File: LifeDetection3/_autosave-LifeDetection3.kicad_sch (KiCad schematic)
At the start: 21 parts, among them J1 Power, J12 XT60PW-M, J2 PWM, J3 Analog, J4 PWM, J5 Analog, J6 Communication, J7 Digital, U1 TLP3545

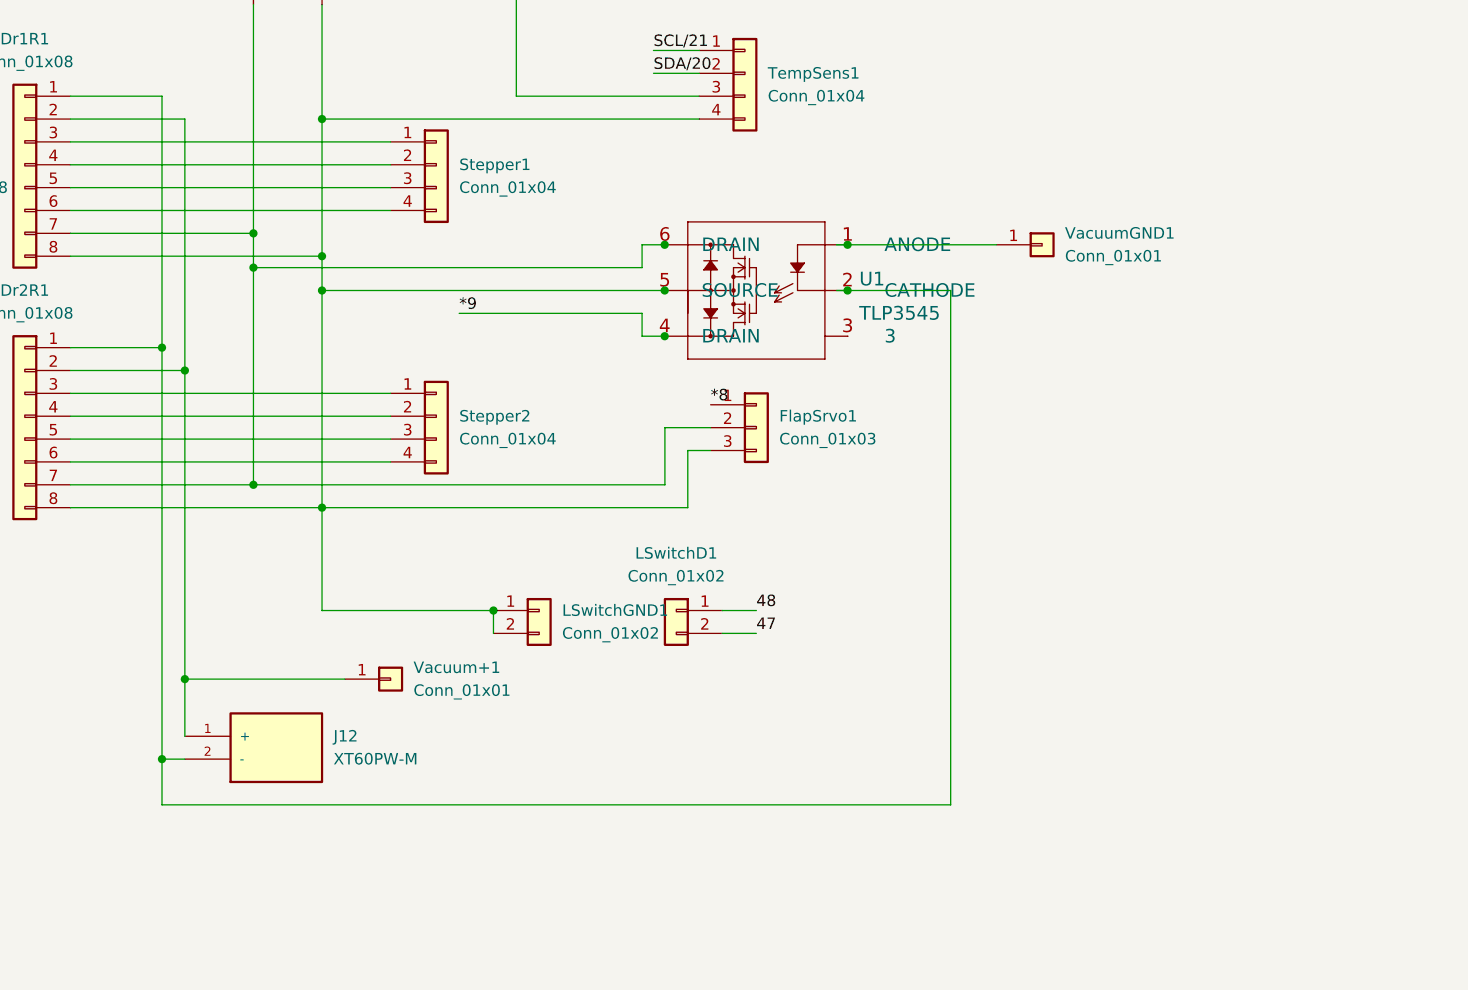
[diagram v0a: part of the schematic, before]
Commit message: more final touches
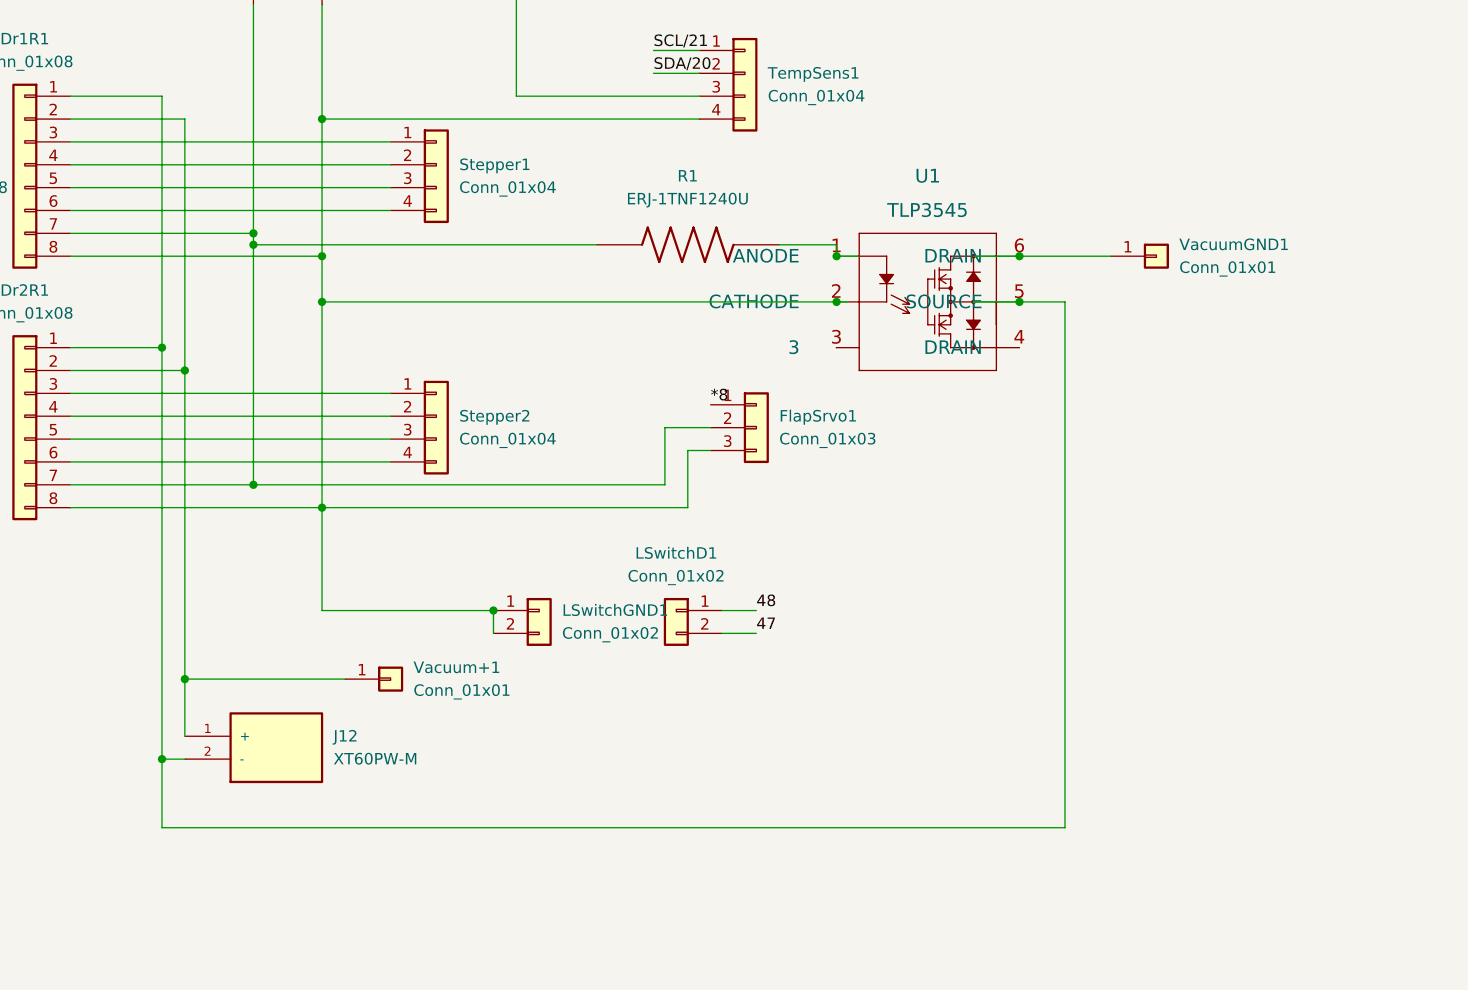
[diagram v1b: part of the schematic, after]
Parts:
- added R1: ERJ-1TNF1240U, ERJ-1TNF1240U(2):RESC6432X70N, symbol ERJ-1TNF1240U:ERJ-1TNF1240U
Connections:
- net *9: no longer U1.4 (DRAIN)
- net +5V: now also R1.1; no longer U1.6 (DRAIN)
- net GND: now also U1.2 (CATHODE); no longer U1.5 (SOURCE)
- net at Dr1R1.1 (Pin_1), Dr2R1.1 (Pin_1), J12.2 (-): now also U1.5 (SOURCE); no longer U1.2 (CATHODE)
- net at U1.1 (ANODE): now also R1.2; no longer VacuumGND1.1 (Pin_1)
- new net: U1.6 (DRAIN), VacuumGND1.1 (Pin_1)
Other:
- moved on the sheet: VacuumGND1
